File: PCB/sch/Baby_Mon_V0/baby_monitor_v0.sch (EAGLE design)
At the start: 2 parts, among them U1 NRF5340-QKAA-AB0-R

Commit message: u
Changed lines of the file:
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@@
 <wire x1="2.54" y1="78.74" x2="2.54" y2="76.2" width="0.1524" layer="91"/>
 <wire x1="2.54" y1="78.74" x2="45.72" y2="78.74" width="0.1524" layer="91"/>
-<wire x1="45.72" y1="78.74" x2="45.72" y2="63.5" width="0.1524" layer="91"/>
 <junction x="2.54" y="78.74"/>
+<wire x1="45.72" y1="63.5" x2="45.72" y2="78.74" width="0.1524" layer="91"/>
 </segment>
 </net>

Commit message: u
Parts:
- added C2, C6: 1uF, SparkFun-Capacitors:CAP0402-CAP
- added C3: 1.0uF, SparkFun-Capacitors:CAP0402-CAP
- added C4, C5, C7: 0.1uF, SparkFun-Capacitors:CAP0402-CAP
- added C8: 0.7pF, SparkFun-Capacitors:CAP0402-CAP
- added FRAME1, FRAME2, FRAME3: FRAME-LETTERNO_PACKAGE, SparkFun-Aesthetics:FRAME-LETTERNO_PACKAGE
- added J10, J11, J7, J8, J9: (no value), graftel-internal-ic:M01TINY
- added L1, L2: 15nH, SparkFun-Passives:INDUCTOR0402
- added L3, L4: 10uH, SparkFun-Passives:INDUCTOR0603
- added L5: 2.2nH, SparkFun-Passives:INDUCTOR0402
- added U2: MAX30101EFD+, graftel-internal-ic:MAX30101EFD+
- added U3: MAX30205MTA+, graftel-internal-ic:MAX30205MTA+
- added X1: XRCGB32M000F2P10R0, graftel-internal-ic:XRCGB32M000F2P10R0
- C1: value (none) -> 1uF; device SparkFun-Capacitors:CAP0603-CAP -> SparkFun-Capacitors:CAP0402-CAP
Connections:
- new net N$1: J11.1, U1G$4.SWDIO
- new net N$10: U1G$4.XC1, X1.2
- new net N$11: U1G$4.XC2, X1.4
- new net N$12: C8.2, L5.2, U1G$4.ANT
- new net N$2: J10.1, U1G$4.SWDCLK
- new net N$3: J9.1, U1G$4.!RESET
- new net N$4: L4.2, U1G$1.DCC
- new net N$5: L1.2, L4.1
- new net N$6: L2.2, L3.1
- new net N$7: L3.2, U1G$1.DCCD
- new net N$8: C2.1, L1.1, U1G$1.DECR, U1G$1.DECRF
- new net N$9: C1.1, L2.1, U1G$1.DECD
- net 3.3V: now also C3.1, C4.1, C5.1, C6.1, C7.1, J8.1, U1G$1.VDD1, U1G$1.VDD2, U1G$1.VDD3; no longer C1.1
- net GND: now also C2.2, C3.2, C4.2, C5.2, C6.2, C7.2, C8.1, J7.1, X1.1, X1.3

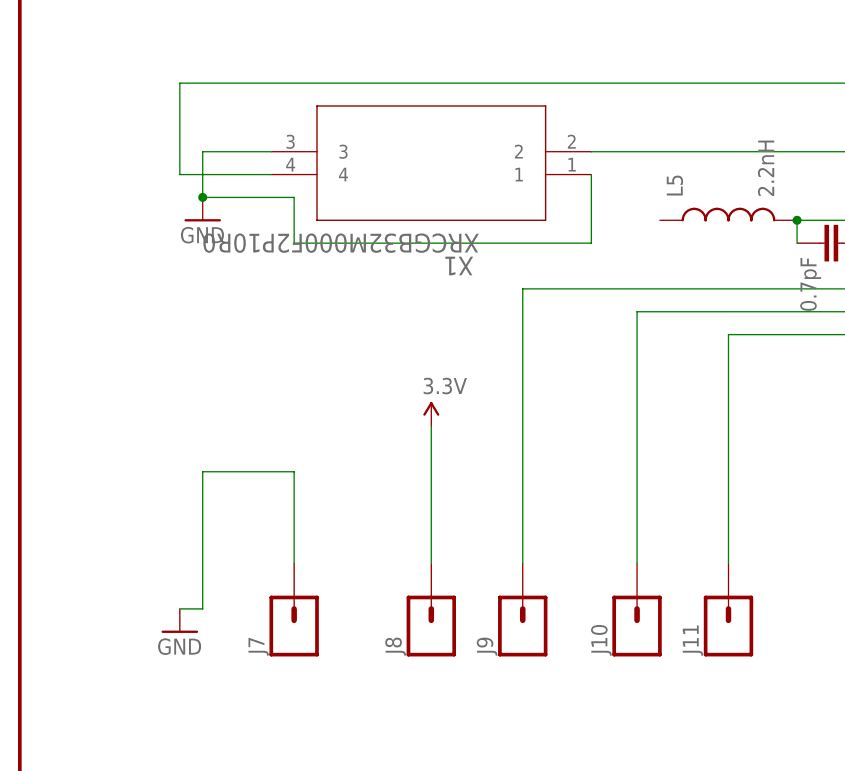
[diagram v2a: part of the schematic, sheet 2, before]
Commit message: u
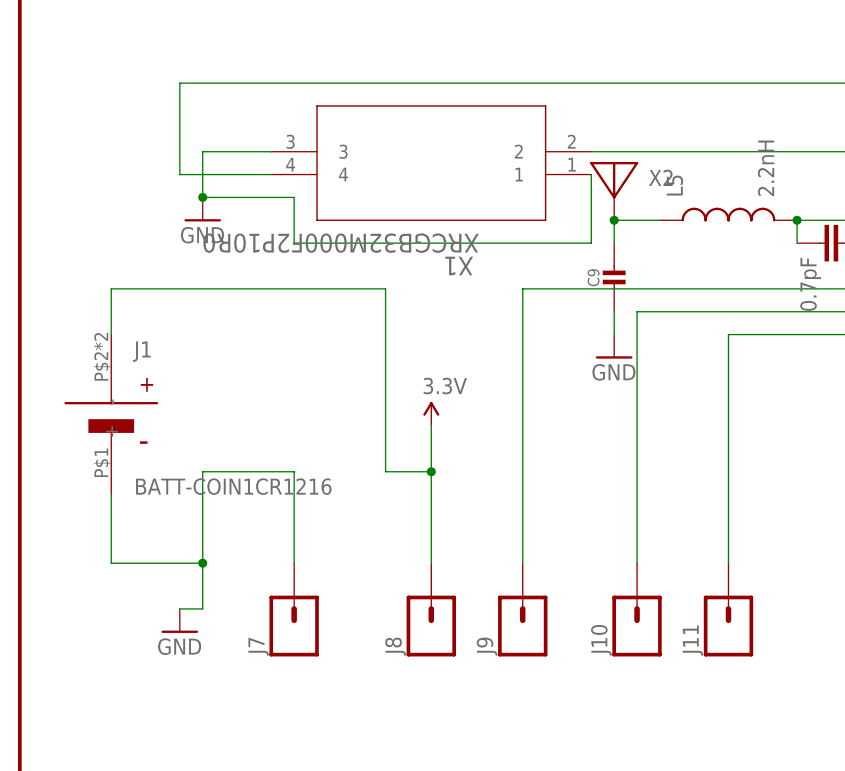
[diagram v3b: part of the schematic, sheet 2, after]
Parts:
- added C9: (no value), graftel-internal-ic:MICROBUILDER_CAP_CERAMIC_0402MP
- added J1: BATT-COIN1CR1216, graftel-internal-ic:BATT-COIN1CR1216
- added X2: (no value), graftel-internal-ic:ADAFRUIT_WIRELESS_ANTENNA_JOHANSON_2450AT18B100
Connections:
- new net N$13: C9.1, L5.1, X2.P$1
- net 3.3V: now also J1.+
- net GND: now also C9.2, J1.-
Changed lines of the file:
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@@
 <layer number="56" name="wert" color="7" fill="1" visible="no" active="no"/>
 <layer number="57" name="tCAD" color="7" fill="1" visible="no" active="no"/>
+<layer number="58" name="bCAD" color="7" fill="1" visible="no" active="no"/>
 <layer number="59" name="tCarbon" color="7" fill="1" visible="no" active="no"/>
 <layer number="60" name="bCarbon" color="7" fill="1" visible="no" active="no"/>
@@
 <layer number="136" name="silktop" color="7" fill="1" visible="yes" active="yes"/>
 <layer number="137" name="silkbottom" color="7" fill="1" visible="yes" active="yes"/>
+<layer number="138" name="EEE" color="7" fill="1" visible="yes" active="yes"/>
+<layer number="139" name="_tKeepout" color="7" fill="1" visible="yes" active="yes"/>
+<layer number="140" name="mbKeepout" color="7" fill="1" visible="yes" active="yes"/>
+<layer number="141" name="ASSEMBLY_TOP" color="7" fill="1" visible="yes" active="yes"/>
+<layer number="142" name="mbRestrict" color="7" fill="1" visible="yes" active="yes"/>
+<layer number="143" name="PLACE_BOUND_TOP" color="7" fill="1" visible="yes" active="yes"/>
 <layer number="144" name="Drill_legend" color="7" fill="1" visible="yes" active="yes"/>
 <layer number="145" name="DrillLegend_01-16" color="7" fill="1" visible="yes" active="yes"/>
 <layer number="146" name="DrillLegend_01-20" color="7" fill="1" visible="yes" active="yes"/>
+<layer number="147" name="PIN_NUMBER" color="7" fill="1" visible="yes" active="yes"/>
+<layer number="148" name="mDocument" color="7" fill="1" visible="yes" active="yes"/>
+<layer number="149" name="DrillLegend_02-15" color="7" fill="1" visible="yes" active="yes"/>
 <layer number="150" name="Notes" color="7" fill="1" visible="yes" active="yes"/>
 <layer number="151" name="HeatSink" color="7" fill="1" visible="yes" active="yes"/>
@@
 <layer number="154" name="FabDoc2" color="7" fill="1" visible="yes" active="yes"/>
 <layer number="155" name="FabDoc3" color="7" fill="1" visible="yes" active="yes"/>
+<layer number="166" name="AntennaArea" color="7" fill="1" visible="yes" active="yes"/>
+<layer number="168" name="4mmHeightArea" color="7" fill="1" visible="yes" active="yes"/>
+<layer number="191" name="mNets" color="7" fill="1" visible="yes" active="yes"/>
+<layer number="192" name="mBusses" color="7" fill="1" visible="yes" active="yes"/>
+<layer number="193" name="mPins" color="7" fill="1" visible="yes" active="yes"/>
+<layer number="194" name="mSymbols" color="7" fill="1" visible="yes" active="yes"/>
+<layer number="195" name="mNames" color="7" fill="1" visible="yes" active="yes"/>
+<layer number="196" name="mValues" color="7" fill="1" visible="yes" active="yes"/>
 <layer number="199" name="Contour" color="7" fill="1" visible="yes" active="yes"/>
 <layer number="200" name="200bmp" color="1" fill="10" visible="yes" active="yes"/>
@@
 <part name="C8" library="SparkFun-Capacitors" deviceset="CAP" device="0402-CAP" value="0.7pF"/>
 <part name="GND7" library="SparkFun-Aesthetics" deviceset="GND" device=""/>
+<part name="J1" library="graftel-internal-ic" deviceset="BATT-COIN1" device="CR1216"/>
+<part name="X2" library="graftel-internal-ic" deviceset="ADAFRUIT_WIRELESS_ANTENNA_JOHANSON_2450AT18B100" device=""/>
+<part name="C9" library="graftel-internal-ic" deviceset="MICROBUILDER_CAP_CERAMIC" device="_0402MP"/>
+<part name="GND8" library="SparkFun-Aesthetics" deviceset="GND" device=""/>
 </parts>
 <sheets>
@@
 <attribute name="VALUE" x="93.98" y="101.6" size="1.778" layer="96"/>
 </instance>
+<instance part="J1" gate="G$1" x="10.16" y="86.36" smashed="yes">
+<attribute name="VALUE" x="12.7" y="78.74" size="1.778" layer="96"/>
+<attribute name="NAME" x="12.7" y="93.98" size="1.778" layer="95"/>
+</instance>
+<instance part="X2" gate="G$1" x="66.04" y="111.76" smashed="yes">
+<attribute name="NAME" x="69.85" y="113.03" size="1.778" layer="95"/>
+<attribute name="VALUE" x="69.85" y="110.49" size="1.778" layer="96"/>
+</instance>
+<instance part="C9" gate="G$1" x="66.04" y="101.6" smashed="yes">
+<attribute name="NAME" x="63.75" y="102.85" size="1.27" layer="95" font="vector" rot="R90" align="center"/>
+<attribute name="VALUE" x="68.34" y="102.85" size="1.27" layer="96" font="vector" rot="R90" align="center"/>
+</instance>
+<instance part="GND8" gate="1" x="66.04" y="93.98" smashed="yes">
+<attribute name="VALUE" x="63.5" y="91.44" size="1.778" layer="96"/>
+</instance>
 </instances>
 <busses>
@@
 <segment>
 <pinref part="SUPPLY2" gate="G$1" pin="3.3V"/>
-<wire x1="45.72" y1="86.36" x2="45.72" y2="71.12" width="0.1524" layer="91"/>
+<wire x1="45.72" y1="86.36" x2="45.72" y2="81.28" width="0.1524" layer="91"/>
 <pinref part="J8" gate="G$1" pin="1"/>
+<pinref part="J1" gate="G$1" pin="+"/>
+<wire x1="45.72" y1="81.28" x2="45.72" y2="71.12" width="0.1524" layer="91"/>
+<wire x1="10.16" y1="96.52" x2="10.16" y2="101.6" width="0.1524" layer="91"/>
+<wire x1="10.16" y1="101.6" x2="40.64" y2="101.6" width="0.1524" layer="91"/>
+<wire x1="40.64" y1="101.6" x2="40.64" y2="81.28" width="0.1524" layer="91"/>
+<wire x1="40.64" y1="81.28" x2="45.72" y2="81.28" width="0.1524" layer="91"/>
+<junction x="45.72" y="81.28"/>
 </segment>
 </net>
@@
 <pinref part="GND2" gate="1" pin="GND"/>
 <wire x1="17.78" y1="66.04" x2="20.32" y2="66.04" width="0.1524" layer="91"/>
-<wire x1="20.32" y1="66.04" x2="20.32" y2="81.28" width="0.1524" layer="91"/>
+<wire x1="20.32" y1="66.04" x2="20.32" y2="71.12" width="0.1524" layer="91"/>
+<wire x1="20.32" y1="71.12" x2="20.32" y2="81.28" width="0.1524" layer="91"/>
 <wire x1="20.32" y1="81.28" x2="30.48" y2="81.28" width="0.1524" layer="91"/>
 <pinref part="J7" gate="G$1" pin="1"/>
 <wire x1="30.48" y1="71.12" x2="30.48" y2="81.28" width="0.1524" layer="91"/>
+<pinref part="J1" gate="G$1" pin="-"/>
+<wire x1="10.16" y1="78.74" x2="10.16" y2="71.12" width="0.1524" layer="91"/>
+<wire x1="10.16" y1="71.12" x2="20.32" y2="71.12" width="0.1524" layer="91"/>
+<junction x="20.32" y="71.12"/>
 </segment>
 <segment>
@@
 <wire x1="93.98" y1="106.68" x2="96.52" y2="106.68" width="0.1524" layer="91"/>
 </segment>
+<segment>
+<pinref part="C9" gate="G$1" pin="2"/>
+<pinref part="GND8" gate="1" pin="GND"/>
+<wire x1="66.04" y1="99.06" x2="66.04" y2="96.52" width="0.1524" layer="91"/>
+</segment>
 </net>
 <net name="N$10" class="0">
@@
 </segment>
 </net>
+<net name="N$13" class="0">
+<segment>
+<pinref part="L5" gate="G$1" pin="1"/>
+<pinref part="X2" gate="G$1" pin="P$1"/>
+<wire x1="71.12" y1="109.22" x2="66.04" y2="109.22" width="0.1524" layer="91"/>
+<pinref part="C9" gate="G$1" pin="1"/>
+<wire x1="66.04" y1="109.22" x2="66.04" y2="106.68" width="0.1524" layer="91"/>
+<junction x="66.04" y="109.22"/>
+</segment>
+</net>
